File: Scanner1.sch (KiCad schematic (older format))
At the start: 45 parts, among them J1 0548190519, J2 Conn_02x05_Odd_Even, J3 Conn_02x03_Odd_Even, Q1 MOSFET_N, SW1 SW_Push, SW2 SW_Push, SW3 SW_Push, U1 ATmega32U4-AU, Y1 16 MHz X322516MLB4SI

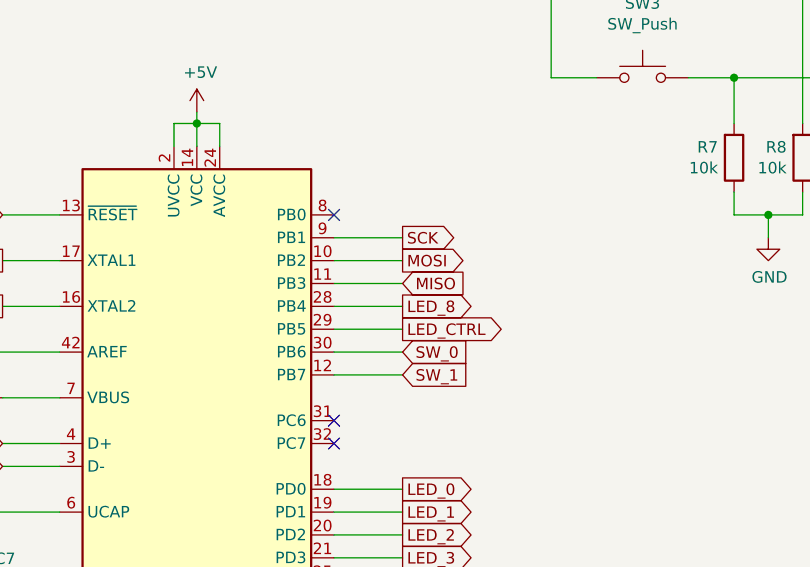
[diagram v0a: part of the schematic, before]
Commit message: More layout
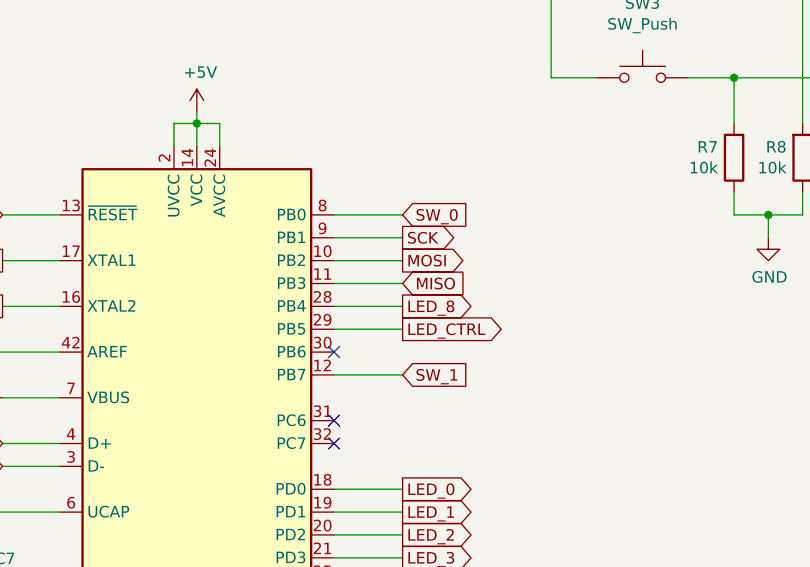
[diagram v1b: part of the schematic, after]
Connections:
- net SW_0: now also U1.8 (PB0); no longer U1.30 (PB6)
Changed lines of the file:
@@
 Wire Wire Line
 	9100 4950 9350 4950
-Text GLabel 6050 3250 2    50   Input ~ 0
+Text GLabel 6050 2650 2    50   Input ~ 0
 SW_0
 Text GLabel 6050 3350 2    50   Input ~ 0
 SW_1
-Wire Wire Line
-	6050 3250 5750 3250
 Wire Wire Line
 	5750 3350 6050 3350
@@
 Wire Wire Line
 	9800 5850 9800 6000
-NoConn ~ 5750 2650
+NoConn ~ 5750 3250
 NoConn ~ 5750 3550
 NoConn ~ 5750 3650
@@
 Text Label 1550 6150 1    50   ~ 0
 VBUS
+Wire Wire Line
+	6050 2650 5750 2650
 $EndSCHEMATC
